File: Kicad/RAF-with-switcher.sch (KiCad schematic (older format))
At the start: 29 parts, among them J1 CONN_01X03, J2 CONN_01X03, J3 SOL, J4 CONN_01X03, J5 PUMP, J6 WS2811-OUT, J7 I2C, P1 Power, P2 Analog, P3 Digital, P4 Digital, Q1 FDC6305N, U1 RGB_WS2811B, U2 LF60CDT

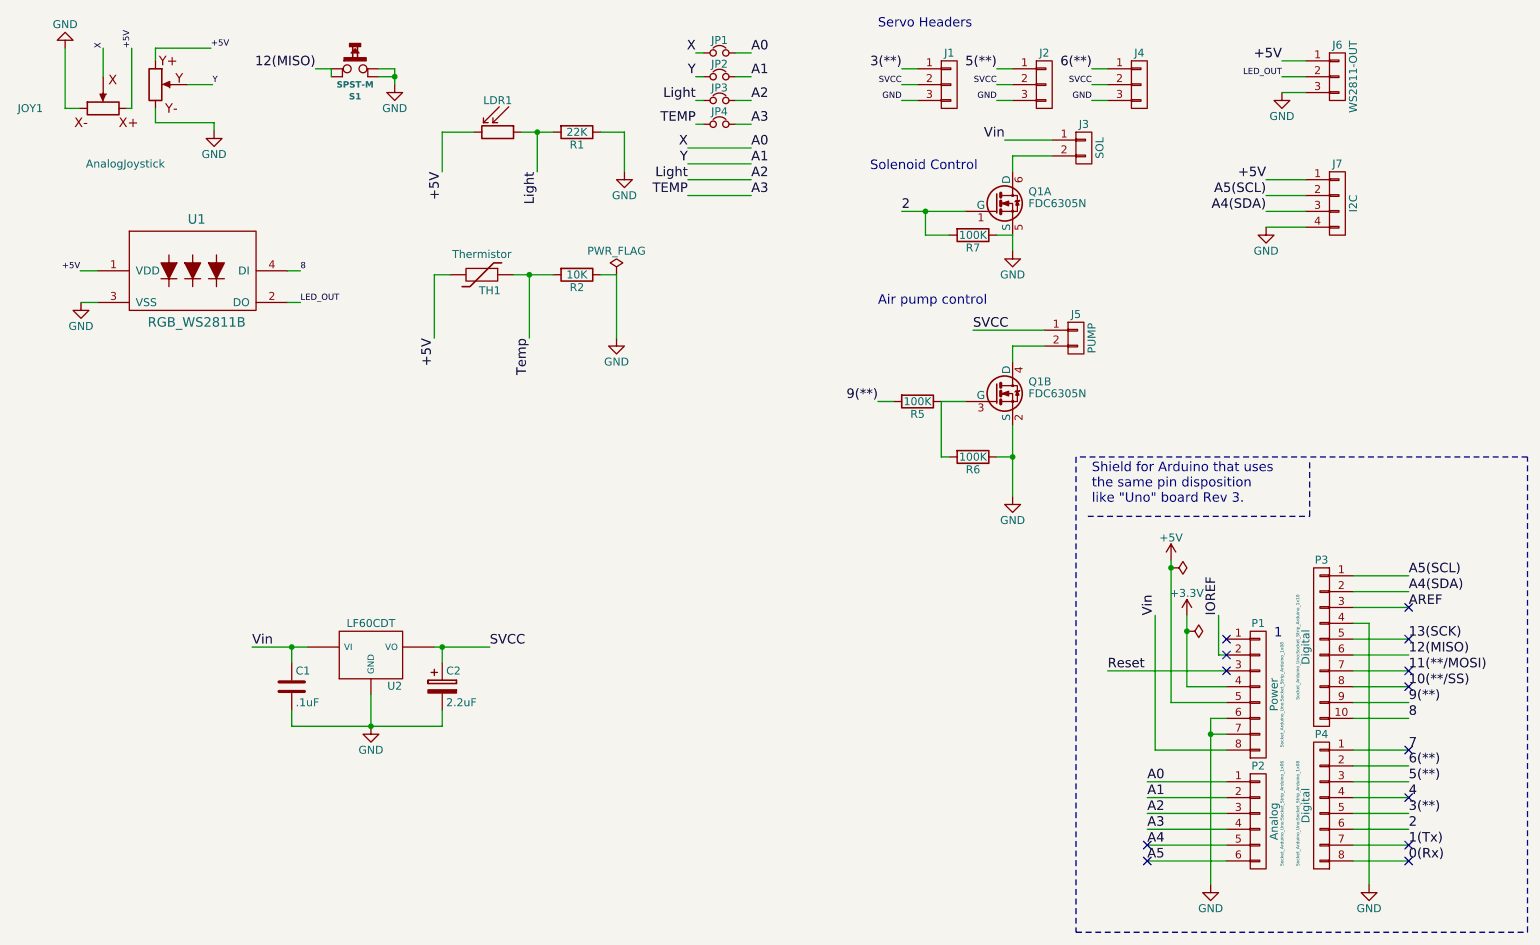
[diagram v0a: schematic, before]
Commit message: new parts, initial layout, backup of switcher design
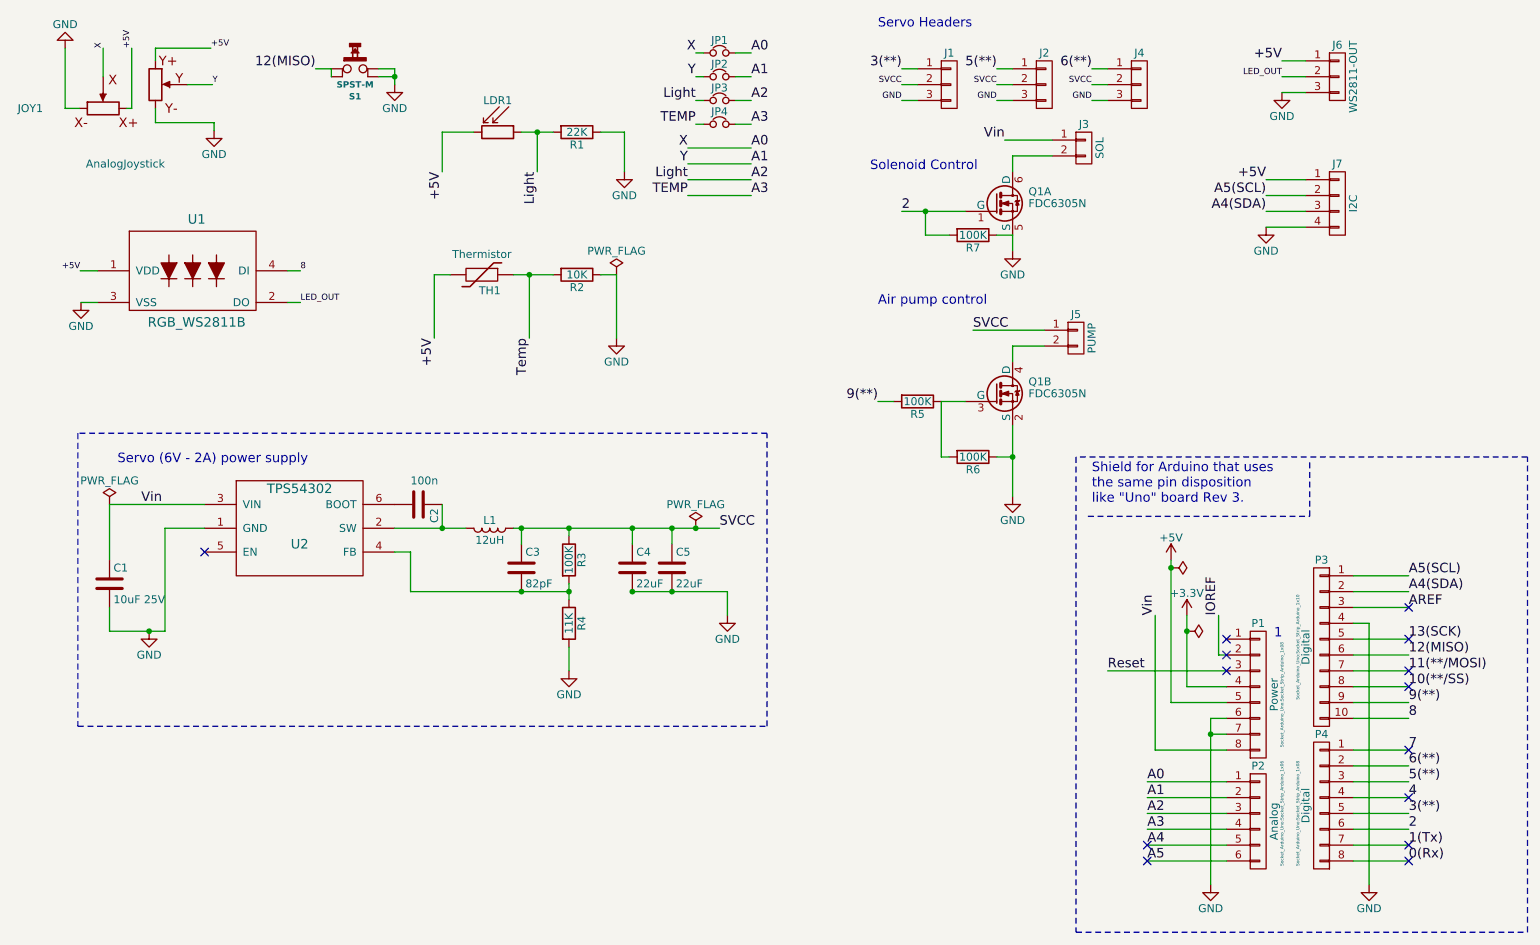
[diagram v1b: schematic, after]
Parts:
- removed C2: 2.2uF, Capacitors_SMD:CP_Elec_4x5.7, symbol CP
- removed U2: LF60CDT, RAF_Libs:DPak, symbol LF60CDT
- added C2: 100n, Resistors_SMD:R_0805_HandSoldering, symbol C
- added C3: 82pF, Resistors_SMD:R_0402, symbol C
- added C4, C5: 22uF, Resistors_SMD:R_1210_HandSoldering, symbol C
- added L1: 12uH, RAF_Libs:ELL-ATV120M, symbol L
- added R3: 100K, Resistors_SMD:R_0805_HandSoldering, symbol R
- added R4: 11K, Resistors_SMD:R_0805_HandSoldering, symbol R
- added U2: TPS54302, TO_SOT_Packages_SMD:SOT-23-6, symbol TPS54302
- C1: value .1uF -> 10uF 25V; footprint Capacitors_SMD:C_0805_HandSoldering -> Resistors_SMD:R_1206_HandSoldering
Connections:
- net GND: now also C4.2, C5.2, R4.2, U2.1 (GND)
- net SVCC: now also C3.1, C4.1, C5.1, L1.1, R3.1
- net Vin: now also U2.3 (VIN)
- new net: C2.1, L1.2, U2.2 (SW)
- new net: C3.2, R3.2, R4.1, U2.4 (FB)
- new net: C2.2, U2.6 (BOOT)
- no-connect marks 13 -> 14
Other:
- note added: "Servo (6V - 2A) power supply"
